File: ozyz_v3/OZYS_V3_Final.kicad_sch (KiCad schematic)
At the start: 26 parts, among them CN1 532610571, J1 5037630491, U1 ISO1044BD, U2 STM32G474CETx, U3 MKDV32GCL-STP, X2 MC-306 32.768kHz 6.0pF 20ppm

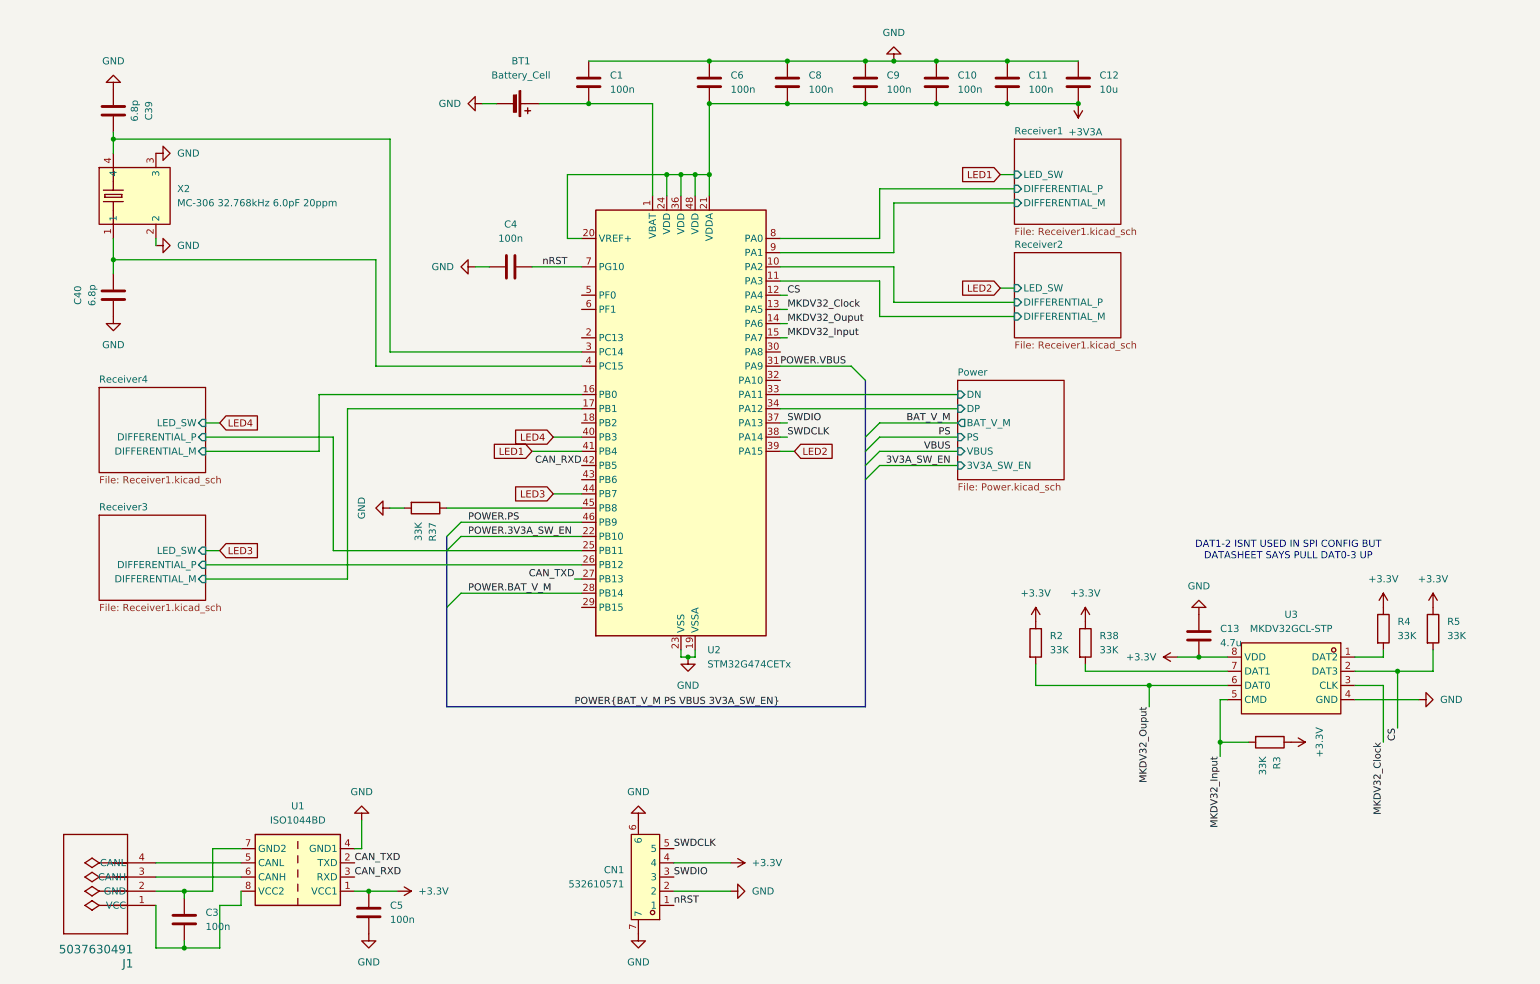
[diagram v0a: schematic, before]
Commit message: OZYS ready for layout
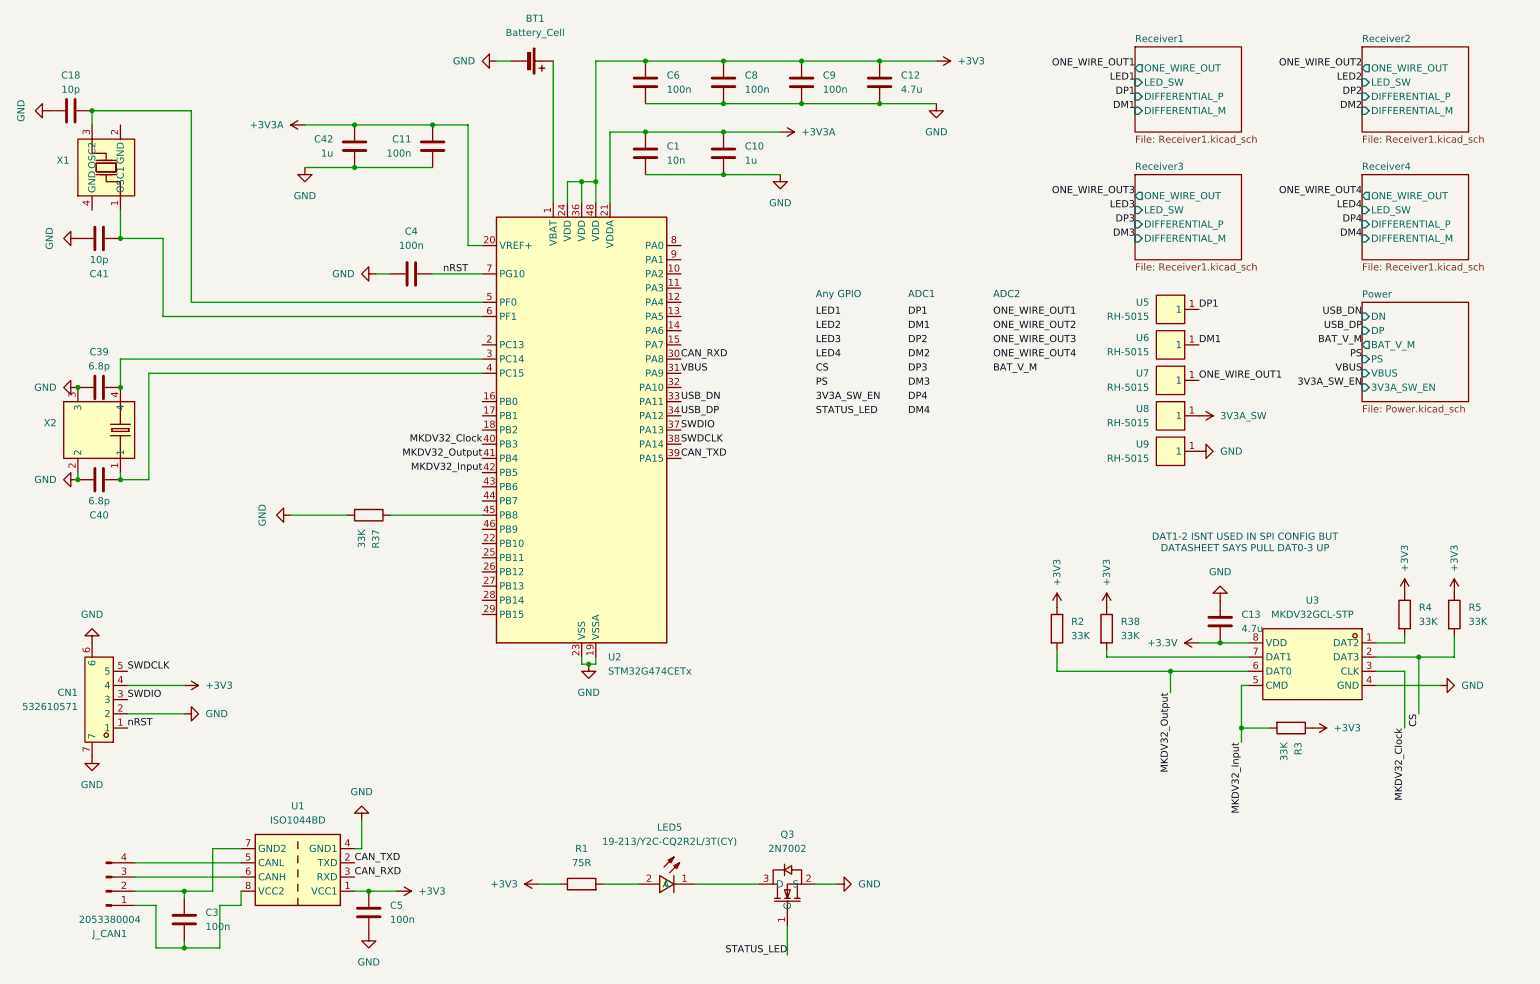
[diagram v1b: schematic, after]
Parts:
- removed J1: 5037630491, symbol Rocketry_Manual:5037630491
- added C18, C41: 10p, Capacitor_SMD:C_0603_1608Metric_Pad1.08x0.95mm_HandSolder, symbol Device:C
- added C42: 1u, Capacitor_SMD:C_0402_1005Metric, symbol Device:C
- added J_CAN1: 2053380004, Rocketry_Manual:CONN_2053380000-SD_04_MOL, symbol Connector:Conn_01x04_Pin
- added LED5: 19-213/Y2C-CQ2R2L/3T(CY), Rocketry_Easyeda:LED0603-RD-YELLOW, symbol Rocketry_Easyeda:19-213_Y2C-CQ2R2L_3T(CY) (0603 Yellow)
- added Q3: 2N7002, Rocketry_Easyeda:SOT-23-3_L2.9-W1.3-P1.90-LS2.4-BR, symbol Rocketry_Easyeda:2N7002
- added R1: 75R, Resistor_SMD:R_0402_1005Metric, symbol Device:R
- added U5, U6, U7, U8, U9: RH-5015, Rocketry_Easyeda:SMD_RH-5015, symbol Rocketry_Easyeda:RH-5015
- added X1: X322516MLB4SI, Rocketry_Easyeda:OSC-SMD_4P-L3.2-W2.5-BL, symbol Rocketry_Easyeda:X322516MLB4SI
- C1: value 100n -> 10n
- C10: value 100n -> 1u
- C12: value 10u -> 4.7u; footprint Capacitor_SMD:C_0603_1608Metric -> Capacitor_SMD:C_0402_1005Metric
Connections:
- net POWER.VBUS is gone; now on net VBUS: U2.31 (PA9)
- net +3.3V: no longer C5.2, CN1.4, R2.1, R3.1, R38.1, R4.1, R5.1, U1.1 (VCC1)
- net +3V3A: now also C1.1, C11.1, C42.2; no longer C11.2, C12.2, C6.2, C8.2, C9.2, U2.24 (VDD), U2.36 (VDD), U2.48 (VDD)
- net CAN_RXD: now also U2.30 (PA8); no longer U2.42 (PB5)
- net CAN_TXD: now also U2.39 (PA15); no longer U2.27 (PB13)
- net CS: no longer U2.12 (PA4)
- net GND: now also C1.2, C11.2, C12.2, C40.2, C6.2, C8.2, C9.2, C18.1, C41.1, C42.1, Q3.2 (S), U9.1; no longer C1.1, C11.1, C12.1, C40.1, C6.1, C8.1, C9.1
- net LED1: no longer U2.41 (PB4)
- net LED2: no longer U2.39 (PA15)
- net LED3: no longer U2.44 (PB7)
- net LED4: no longer U2.40 (PB3)
- net MKDV32_Clock: now also U2.40 (PB3); no longer U2.13 (PA5)
- net MKDV32_Input: now also U2.42 (PB5); no longer U2.15 (PA7)
- net at BT1.1 (+), U2.1 (VBAT): no longer C1.2
- net at U2.4 (PC15), X2.1: now also C40.1; no longer C40.2
- net at U2.5 (PF0): now also C18.2, X1.3 (OSC2)
- net at U2.6 (PF1): now also C41.2, X1.1 (OSC1)
- net at C3.2, U1.8 (VCC2): now also J_CAN1.1 (Pin_1)
- net at C3.1, U1.7 (GND2): now also J_CAN1.2 (Pin_2)
- net at U1.6 (CANH): now also J_CAN1.3 (Pin_3)
- net at U1.5 (CANL): now also J_CAN1.4 (Pin_4)
- net MKDV32_Ouput renamed MKDV32_Output
- net MKDV32_Output: now also U2.41 (PB4); no longer U2.14 (PA6)
- net POWER.3V3A_SW_EN: no longer names the net of U2.22 (PB10)
- net POWER.BAT_V_M: no longer names the net of U2.28 (PB14)
- net POWER.PS: no longer names the net of U2.46 (PB9)
- net Power/DN renamed USB_DN
- net Power/DP renamed USB_DP
- net Receiver1/DIFFERENTIAL_M: no longer names the net of U2.9 (PA1)
- net Receiver1/DIFFERENTIAL_P: no longer names the net of U2.8 (PA0)
- net Receiver2/DIFFERENTIAL_M: no longer names the net of U2.11 (PA3)
- net Receiver2/DIFFERENTIAL_P: no longer names the net of U2.10 (PA2)
- net Receiver3/DIFFERENTIAL_M: no longer names the net of U2.17 (PB1)
- net Receiver3/DIFFERENTIAL_P: no longer names the net of U2.26 (PB12)
- net Receiver4/DIFFERENTIAL_M: no longer names the net of U2.16 (PB0)
- net Receiver4/DIFFERENTIAL_P: no longer names the net of U2.25 (PB11)
- new net: LED5.1 (C), Q3.3 (D)
- new net: LED5.2 (A), R1.2
- new net +3V3: C12.1, C5.2, C6.1, C8.1, C9.1, CN1.4, R1.1, R2.1, R3.1, R38.1, R4.1, R5.1, U1.1 (VCC1), U2.24 (VDD), U2.36 (VDD), U2.48 (VDD)
- new net 3V3A_SW: U8.1
- new net DM1: U6.1
- new net DP1: U5.1
- new net ONE_WIRE_OUT1: U7.1
- new net STATUS_LED: Q3.1 (G)
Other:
- sheet Receiver1 ports: added ONE_WIRE_OUT; removed none
- sheet Receiver2 ports: added ONE_WIRE_OUT; removed none
- sheet Receiver3 ports: added ONE_WIRE_OUT; removed none
- sheet Receiver4 ports: added ONE_WIRE_OUT; removed none
- note added: "ADC1"
- note added: "ADC2"
- note added: "Any GPIO"
- moved on the sheet: BT1, C12, C13, C39, C4, C40, C6, C8, C9, CN1, R2, R3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
